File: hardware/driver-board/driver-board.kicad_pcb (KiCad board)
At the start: 2 copper layers, 54 parts, among them J1 Conn_01x10_Male, U1 TXS0108E, U2 ME6210, U3 ME6210, U4 TLV61046ADB, U5 NC7SZ125, U6 FT813, U7 ER-TFT040-2, X1 YSX321SL

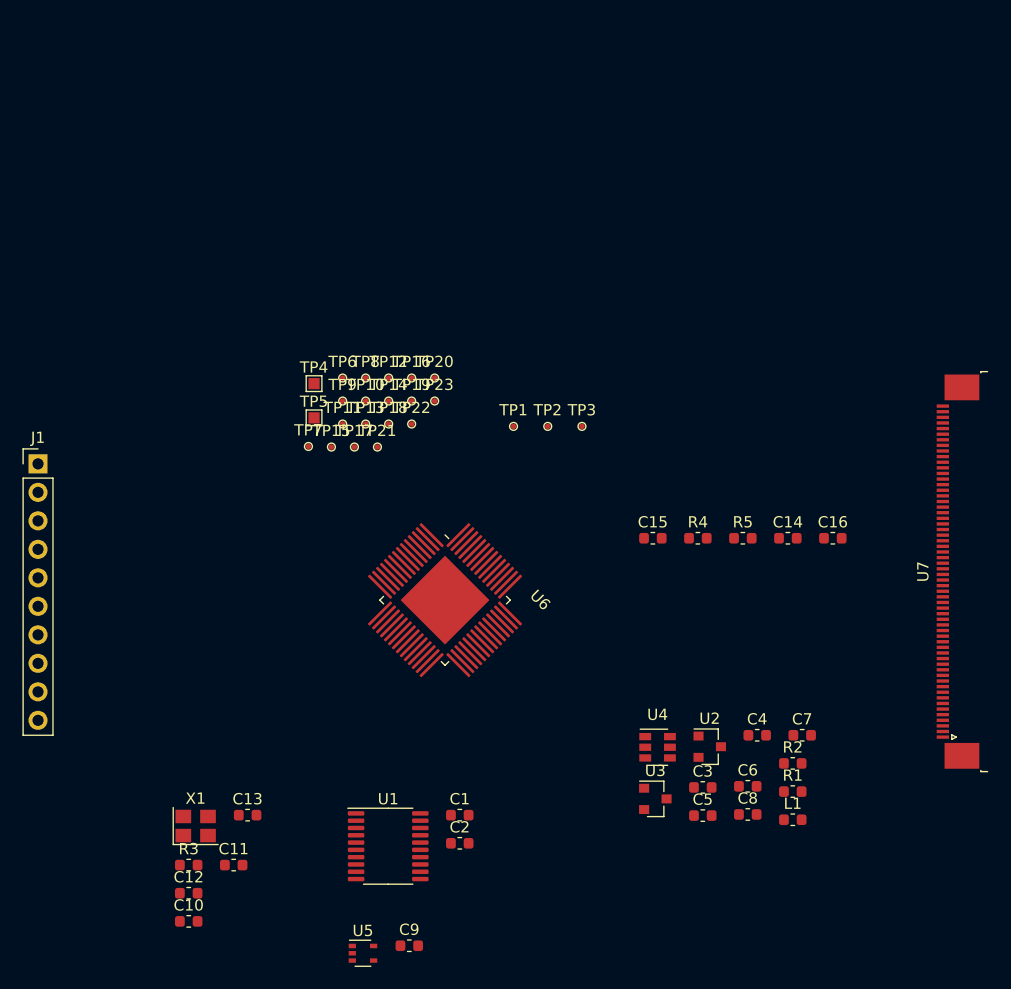
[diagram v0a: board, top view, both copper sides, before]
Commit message: PCB layout on work
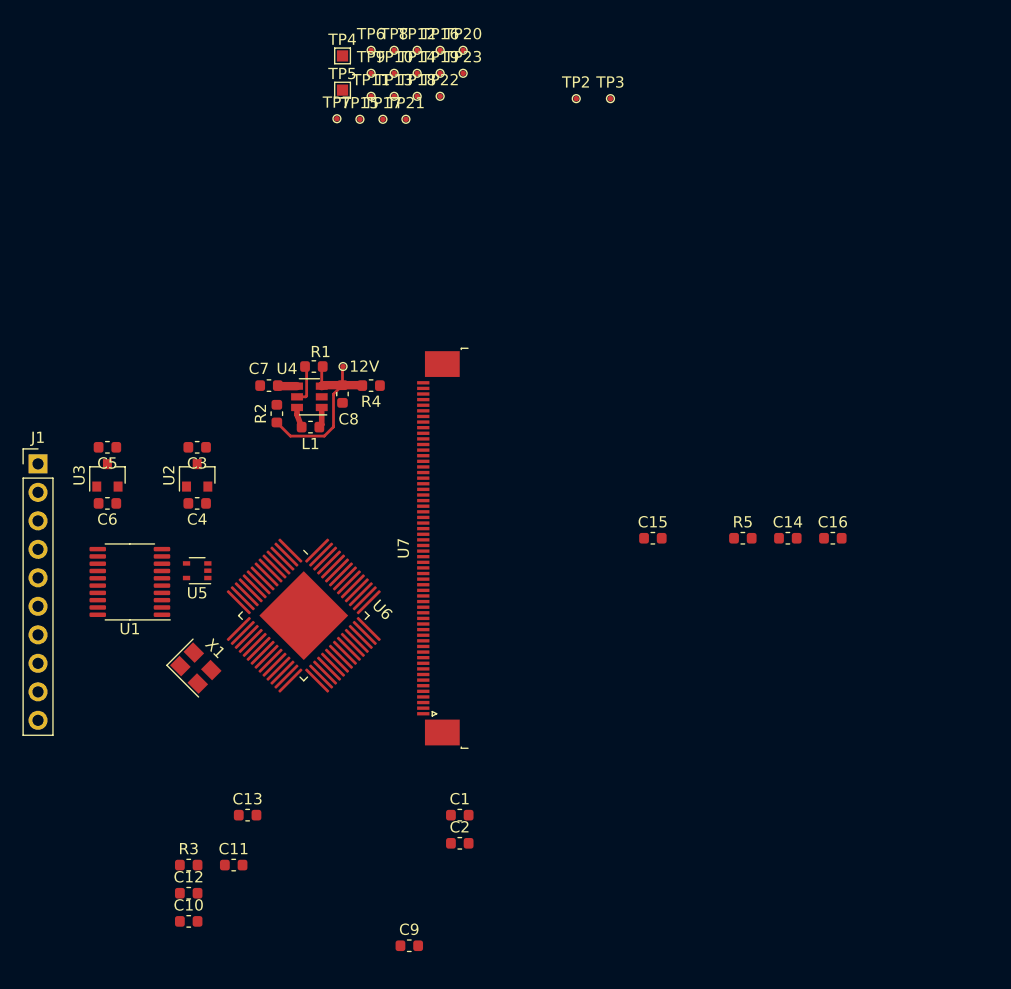
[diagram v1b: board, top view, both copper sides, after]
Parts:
- removed TP1: TestPoint, TestPoint:TestPoint_Pad_D0.5mm
- added 12V: TestPoint, TestPoint:TestPoint_Pad_D0.5mm, F.Cu at (139.5, 50.3)
- moved C5 62.4 mm to (118.5, 57.5), turned to 180 degrees
- moved C6 62.4 mm to (118.5, 62.5), turned to 180 degrees
- moved R1 57.1 mm to (136.9, 50.3), turned to 180 degrees
- moved C7 56.8 mm to (132.9, 52.0), turned to 180 degrees
- moved U3 56.7 mm to (118.5, 60.0), turned to 90 degrees
- moved R2 55.6 mm to (133.6, 54.5), turned to 90 degrees
- moved L1 55.4 mm to (136.6, 55.7)
- moved C3 54.3 mm to (126.5, 57.5), turned to 180 degrees
- moved C4 54.0 mm to (126.5, 62.5), turned to 180 degrees
- moved C8 52.1 mm to (139.4, 52.8), turned to 270 degrees
- moved U2 51.7 mm to (126.5, 60.0), turned to 90 degrees
- moved U7 46.4 mm to (148.0, 66.5)
- moved U4 44.0 mm to (136.5, 53.0), turned to 180 degrees
- moved U5 37.2 mm to (126.5, 68.5), turned to 180 degrees
- moved U1 32.9 mm to (120.5, 69.5), turned to 180 degrees
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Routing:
- net +12V: track 0.00 -> 17.1 mm
- net Net-(R1-Pad2): track 0.00 -> 3.57 mm
- net +5V: track 0.00 -> 3.56 mm
- net Net-(L1-Pad2): track 0.00 -> 1.84 mm
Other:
- copper layers 2 -> 4
- net class Default: trace_width 0.25 -> 0.2; via_dia 0.8 -> 0.45; via_drill 0.4 -> 0.2
- rule via_min_drill: 0.3 -> 0.2
- rule via_min_size: 0.4 -> 0.45
